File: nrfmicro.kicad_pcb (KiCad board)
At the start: 2 copper layers, 18 x 33.3 mm, 24 parts, among them J1 USB_OTG, J2 Serial Connector, J3 Conn_01x02, J4 USB_C_Receptacle_USB2.0, Q1 DMG2305, SW1 SW_SPDT, U2 ProMicro, U3 AP2112K-3.3, U4 MCP73831-2-OT, U5 E73-2G4M08S1C-52840, Y2 32,768

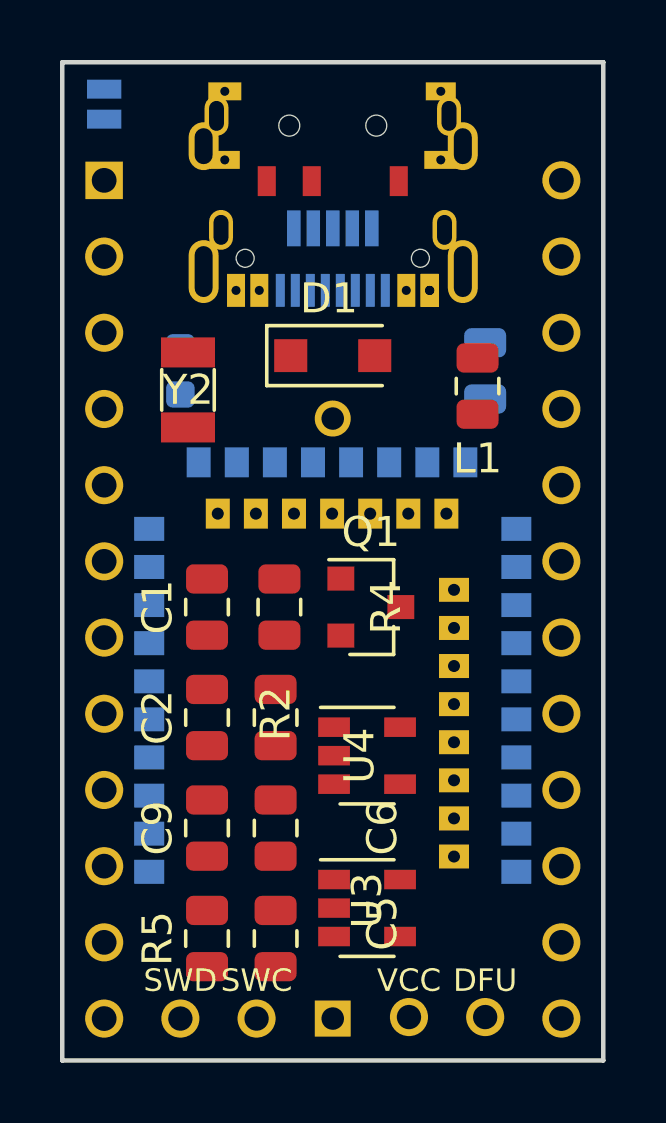
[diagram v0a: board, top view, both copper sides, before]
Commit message: second commit
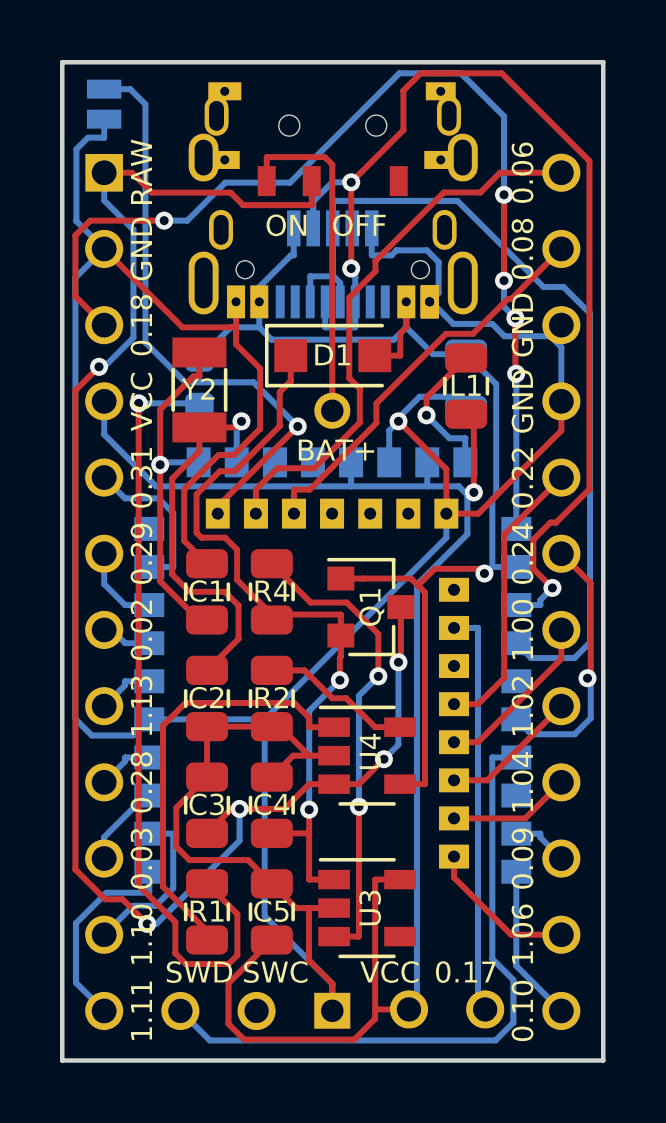
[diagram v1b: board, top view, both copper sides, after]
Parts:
- removed C6, C9: 10uF, Capacitor_SMD:C_0805_2012Metric
- removed D3: LED, LED_SMD:LED_0603_1608Metric
- removed R5: 100K, Resistor_SMD:R_0805_2012Metric
- added C3: 10uF, Capacitor_SMD:C_0805_2012Metric, F.Cu at (99.6, 133.4)
- added C4: 10uF, Capacitor_SMD:C_0805_2012Metric, F.Cu at (101.8, 133.4)
- added D2: LED, LED_SMD:LED_0603_1608Metric, B.Cu at (99.4, 119.3)
- added R1: 1K, Resistor_SMD:R_0805_2012Metric, F.Cu at (99.6, 137.0)
- J2: value Serial Connector -> USB_C_Receptacle_USB2.0; footprint nrfmicro:connector_swd -> nrfmicro:usb_type_c; moved to B.Cu
- J3: value Conn_01x02 -> Serial Connector; footprint nrfmicro:battery_holder_bs-7 -> nrfmicro:connector_swd
- J4: value USB_C_Receptacle_USB2.0 -> Conn_01x02; footprint nrfmicro:usb_type_c -> nrfmicro:battery_holder_bs-7
- R2: value 100K -> 4.7K
- R3: value 1K -> 100K
- R4: value 4.7K -> 100K
- U5: value E73-2G4M08S1C-52840 -> nRF52840
- moved J2 31.4 mm to (103.8, 109.2), turned to 180 degrees
- moved J4 24.1 mm to (103.8, 132.9)
- moved J3 7.11 mm to (103.8, 140.3)
- moved C5 0.90 mm to (101.8, 137.0)
- moved R3 0.74 mm to (108.2, 119.3)
- moved R2 0.65 mm to (101.8, 129.9)
- moved C2 0.64 mm to (99.6, 129.9)
- moved R4 0.57 mm to (101.8, 126.3)
- moved C1 0.51 mm to (99.6, 126.3)
- moved Y2 0.38 mm to (99.4, 119.6)
- moved L1 0.38 mm to (108.2, 119.5)
- moved U2 0.25 mm to (103.8, 124.8)
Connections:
- C5 pad 1: Net-(C5-Pad1) -> VCC
- D1 pad 1: Net-(C5-Pad1) -> Net-(C4-Pad1)
- J3 pad 1: Net-(J3-Pad1) -> SWDIO
- J3 pad 2: GND -> SWDCLK
- Q1 pad 2: Net-(C5-Pad1) -> Net-(C4-Pad1)
- R2 pad 1: VBUS -> Net-(R2-Pad1)
- R3 pad 1: Net-(D3-Pad1) -> VBUS
- R3 pad 2: Net-(R3-Pad2) -> GND
- R4 pad 1: Net-(R4-Pad1) -> Net-(C4-Pad1)
- R4 pad 2: GND -> Net-(R4-Pad2)
- SW1 pad 3: Net-(J3-Pad1) -> Net-(J4-Pad1)
- U3 pad 1: Net-(C5-Pad1) -> Net-(C4-Pad1)
- U3 pad 3: Net-(R5-Pad2) -> Net-(R4-Pad2)
- U4 pad 1: Net-(R3-Pad2) -> Net-(R1-Pad2)
- U4 pad 5: Net-(R4-Pad1) -> Net-(R2-Pad1)
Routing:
- net GND: track 0.00 -> 111.1 mm, vias 0 -> 1
- net VBAT: track 0.00 -> 53.4 mm, vias 0 -> 5
- net VCC: track 0.00 -> 52.0 mm, vias 0 -> 1
- net VBUS: track 0.00 -> 38.9 mm, vias 0 -> 1
- net DATA-: track 0.00 -> 37.5 mm, vias 0 -> 3
- net RESET: track 0.00 -> 34.4 mm, vias 0 -> 5
- net DATA+: track 0.00 -> 29.0 mm
- net Net-(D2-Pad1): track 0.00 -> 26.0 mm, vias 0 -> 1
- net Net-(C4-Pad1): track 0.00 -> 25.5 mm, vias 0 -> 2
- net SWDIO: track 0.00 -> 21.7 mm
- net /P0.26: track 0.00 -> 19.8 mm, vias 0 -> 1
- net TXD: track 0.00 -> 18.5 mm
- net Net-(R4-Pad2): track 0.00 -> 15.7 mm, vias 0 -> 2
- net Net-(R1-Pad2): track 0.00 -> 14.3 mm
- net SWO: track 0.00 -> 13.6 mm
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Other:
- board text added: "OFF"
- board text added: "ON"
